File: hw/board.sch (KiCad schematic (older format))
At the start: 4 parts, among them SW1 SW_PUSH

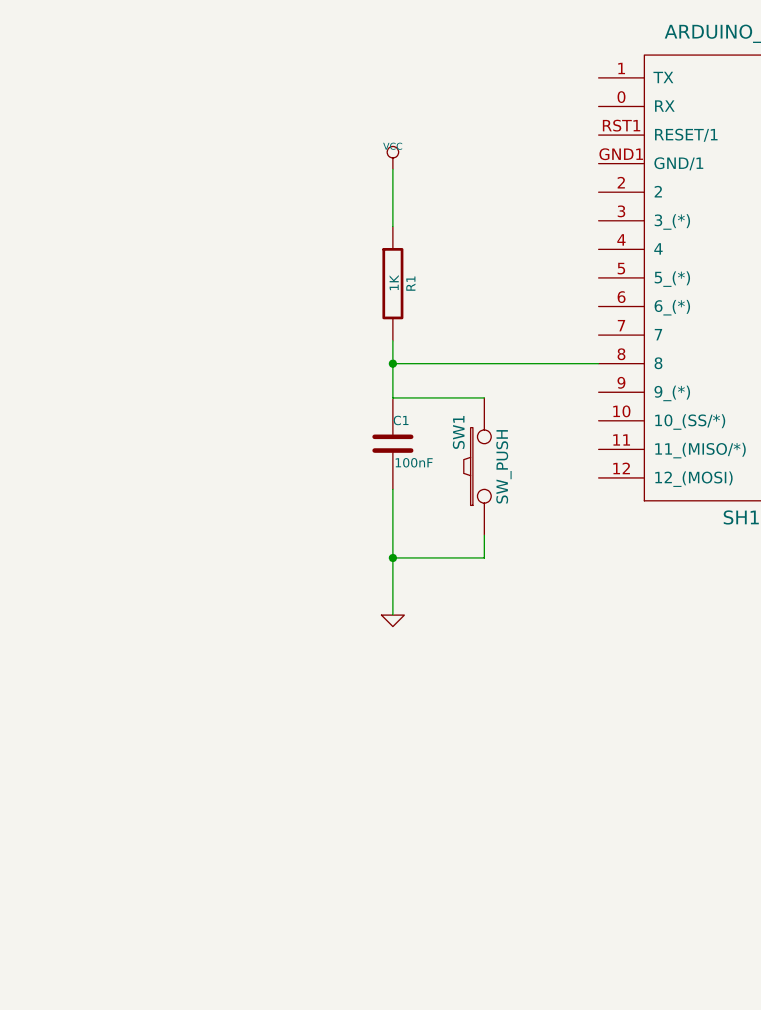
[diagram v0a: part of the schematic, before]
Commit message: Schematic update
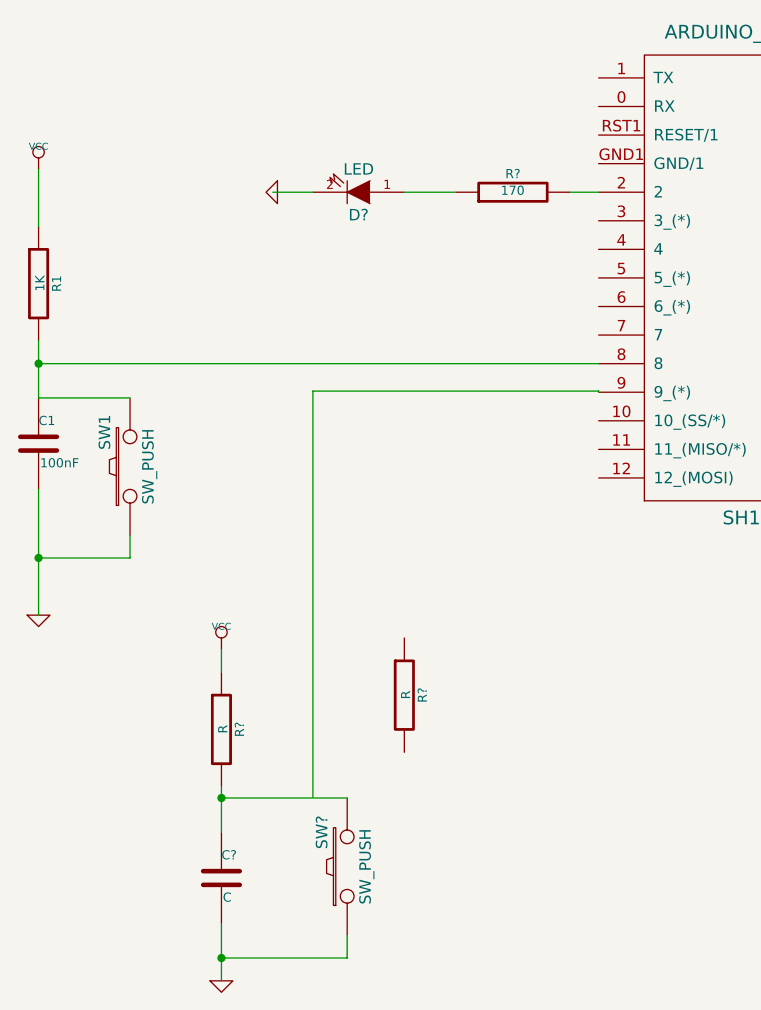
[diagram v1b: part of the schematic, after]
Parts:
- added C?: C, ~, symbol C
- added D?: LED, ~, symbol LED
- added R? (x2): R, ~, symbol R
- added R?: 170, ~, symbol R
- added SW?: SW_PUSH, ~, symbol SW_PUSH
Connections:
- wire segments 7 -> 19
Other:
- moved on the sheet: C1, R1, SW1
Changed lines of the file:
@@
 EESchema Schematic File Version 2
+LIBS:shield_arduino
 LIBS:power
 LIBS:device
@@
 LIBS:contrib
 LIBS:valves
-LIBS:shield_arduino
+LIBS:board-cache
 EELAYER 27 0
 EELAYER END
@@
 Sheet 1 1
 Title ""
-Date "19 sep 2015"
+Date "21 sep 2015"
 Rev ""
 Comp ""
@@
 L R R1
 U 1 1 55FD3C19
-P 3900 3750
-F 0 "R1" V 3980 3750 40  0000 C CNN
-F 1 "1K" V 3907 3751 40  0000 C CNN
-F 2 "~" V 3830 3750 30  0000 C CNN
-F 3 "~" H 3900 3750 30  0000 C CNN
-	1    3900 3750
+P 2350 3750
+F 0 "R1" V 2430 3750 40  0000 C CNN
+F 1 "1K" V 2357 3751 40  0000 C CNN
+F 2 "~" V 2280 3750 30  0000 C CNN
+F 3 "~" H 2350 3750 30  0000 C CNN
+	1    2350 3750
 	1    0    0    -1
 $EndComp
@@
 L C C1
 U 1 1 55FD3C28
-P 3900 4450
-F 0 "C1" H 3900 4550 40  0000 L CNN
-F 1 "100nF" H 3906 4365 40  0000 L CNN
-F 2 "~" H 3938 4300 30  0000 C CNN
-F 3 "~" H 3900 4450 60  0000 C CNN
-	1    3900 4450
+P 2350 4450
+F 0 "C1" H 2350 4550 40  0000 L CNN
+F 1 "100nF" H 2356 4365 40  0000 L CNN
+F 2 "~" H 2388 4300 30  0000 C CNN
+F 3 "~" H 2350 4450 60  0000 C CNN
+	1    2350 4450
 	1    0    0    -1
 $EndComp
@@
 L SW_PUSH SW1
 U 1 1 55FD3C5B
-P 4300 4550
-F 0 "SW1" H 4450 4660 50  0000 C CNN
-F 1 "SW_PUSH" H 4300 4470 50  0000 C CNN
-F 2 "~" H 4300 4550 60  0000 C CNN
-F 3 "~" H 4300 4550 60  0000 C CNN
-	1    4300 4550
+P 2750 4550
+F 0 "SW1" H 2900 4660 50  0000 C CNN
+F 1 "SW_PUSH" H 2750 4470 50  0000 C CNN
+F 2 "~" H 2750 4550 60  0000 C CNN
+F 3 "~" H 2750 4550 60  0000 C CNN
+	1    2750 4550
 	0    -1   -1   0
 $EndComp
@@
 L GND #PWR2
 U 1 1 55FD3C70
-P 3900 5200
-F 0 "#PWR2" H 3900 5200 30  0001 C CNN
-F 1 "GND" H 3900 5130 30  0001 C CNN
-F 2 "" H 3900 5200 60  0000 C CNN
-F 3 "" H 3900 5200 60  0000 C CNN
-	1    3900 5200
+P 2350 5200
+F 0 "#PWR2" H 2350 5200 30  0001 C CNN
+F 1 "GND" H 2350 5130 30  0001 C CNN
+F 2 "" H 2350 5200 60  0000 C CNN
+F 3 "" H 2350 5200 60  0000 C CNN
+	1    2350 5200
 	1    0    0    -1
 $EndComp
@@
 L VCC #PWR1
 U 1 1 55FD3C7F
-P 3900 3250
-F 0 "#PWR1" H 3900 3350 30  0001 C CNN
-F 1 "VCC" H 3900 3350 30  0000 C CNN
-F 2 "" H 3900 3250 60  0000 C CNN
-F 3 "" H 3900 3250 60  0000 C CNN
-	1    3900 3250
-	1    0    0    -1
-$EndComp
-Wire Wire Line
-	4300 4250 3900 4250
-Wire Wire Line
-	3900 4250 3900 4000
-Wire Wire Line
-	3900 3500 3900 3250
-Wire Wire Line
-	3900 4650 3900 5200
-Wire Wire Line
-	4300 4850 4300 4950
-Wire Wire Line
-	4300 4950 3900 4950
-Connection ~ 3900 4950
-Wire Wire Line
-	4800 4100 3900 4100
-Connection ~ 3900 4100
+P 2350 3250
+F 0 "#PWR1" H 2350 3350 30  0001 C CNN
+F 1 "VCC" H 2350 3350 30  0000 C CNN
+F 2 "" H 2350 3250 60  0000 C CNN
+F 3 "" H 2350 3250 60  0000 C CNN
+	1    2350 3250
+	1    0    0    -1
+$EndComp
+Wire Wire Line
+	2750 4250 2350 4250
+Wire Wire Line
+	2350 4250 2350 4000
+Wire Wire Line
+	2350 3500 2350 3250
+Wire Wire Line
+	2350 4650 2350 5200
+Wire Wire Line
+	2750 4850 2750 4950
+Wire Wire Line
+	2750 4950 2350 4950
+Connection ~ 2350 4950
+Connection ~ 2350 4100
+Wire Wire Line
+	2350 4100 4800 4100
+$Comp
+L R R?
+U 1 1 55FFADEF
+P 3950 5550
+F 0 "R?" V 4030 5550 40  0000 C CNN
+F 1 "R" V 3957 5551 40  0000 C CNN
+F 2 "~" V 3880 5550 30  0000 C CNN
+F 3 "~" H 3950 5550 30  0000 C CNN
+	1    3950 5550
+	1    0    0    -1
+$EndComp
+$Comp
+L R R?
+U 1 1 55FFADFE
+P 3150 5700
+F 0 "R?" V 3230 5700 40  0000 C CNN
+F 1 "R" V 3157 5701 40  0000 C CNN
+F 2 "~" V 3080 5700 30  0000 C CNN
+F 3 "~" H 3150 5700 30  0000 C CNN
+	1    3150 5700
+	1    0    0    -1
+$EndComp
+$Comp
+L C C?
+U 1 1 55FFAE0D
+P 3150 6350
+F 0 "C?" H 3150 6450 40  0000 L CNN
+F 1 "C" H 3156 6265 40  0000 L CNN
+F 2 "~" H 3188 6200 30  0000 C CNN
+F 3 "~" H 3150 6350 60  0000 C CNN
+	1    3150 6350
+	1    0    0    -1
+$EndComp
+$Comp
+L SW_PUSH SW?
+U 1 1 55FFAE33
+P 3700 6300
+F 0 "SW?" H 3850 6410 50  0000 C CNN
+F 1 "SW_PUSH" H 3700 6220 50  0000 C CNN
+F 2 "~" H 3700 6300 60  0000 C CNN
+F 3 "~" H 3700 6300 60  0000 C CNN
+	1    3700 6300
+	0    -1   -1   0
+$EndComp
+$Comp
+L VCC #PWR?
+U 1 1 55FFAE77
+P 3150 5350
+F 0 "#PWR?" H 3150 5450 30  0001 C CNN
+F 1 "VCC" H 3150 5450 30  0000 C CNN
+F 2 "" H 3150 5350 60  0000 C CNN
+F 3 "" H 3150 5350 60  0000 C CNN
+	1    3150 5350
+	1    0    0    -1
+$EndComp
+$Comp
+L GND #PWR?
+U 1 1 55FFAE8C
+P 3150 6800
+F 0 "#PWR?" H 3150 6800 30  0001 C CNN
+F 1 "GND" H 3150 6730 30  0001 C CNN
+F 2 "" H 3150 6800 60  0000 C CNN
+F 3 "" H 3150 6800 60  0000 C CNN
+	1    3150 6800
+	1    0    0    -1
+$EndComp
+Wire Wire Line
+	3150 5350 3150 5450
+Wire Wire Line
+	3150 5950 3150 6150
+Wire Wire Line
+	3150 6550 3150 6800
+Wire Wire Line
+	3700 6000 3150 6000
+Connection ~ 3150 6000
+Wire Wire Line
+	3700 6600 3700 6700
+Wire Wire Line
+	3700 6700 3150 6700
+Connection ~ 3150 6700
+Wire Wire Line
+	3550 5995 3550 4220
+Wire Wire Line
+	3550 4220 4800 4220
+Wire Wire Line
+	4800 4220 4800 4225
+$Comp
+L GND #PWR?
+U 1 1 55FFAFE2
+P 3395 3350
+F 0 "#PWR?" H 3395 3350 30  0001 C CNN
+F 1 "GND" H 3395 3280 30  0001 C CNN
+F 2 "" H 3395 3350 60  0000 C CNN
+F 3 "" H 3395 3350 60  0000 C CNN
+	1    3395 3350
+	0    1    1    0
+$EndComp
+$Comp
+L LED D?
+U 1 1 55FFB090
+P 3750 3350
+F 0 "D?" H 3750 3450 50  0000 C CNN
+F 1 "LED" H 3750 3250 50  0000 C CNN
+F 2 "~" H 3750 3350 60  0000 C CNN
+F 3 "~" H 3750 3350 60  0000 C CNN
+	1    3750 3350
+	-1   0    0    1
+$EndComp
+$Comp
+L R R?
+U 1 1 55FFB09F
+P 4425 3350
+F 0 "R?" V 4505 3350 40  0000 C CNN
+F 1 "170" V 4432 3351 40  0000 C CNN
+F 2 "~" V 4355 3350 30  0000 C CNN
+F 3 "~" H 4425 3350 30  0000 C CNN
+	1    4425 3350
+	0    -1   -1   0
+$EndComp
+Wire Wire Line
+	4800 3350 4675 3350
+Wire Wire Line
+	4175 3350 3950 3350
+Wire Wire Line
+	3375 3350 3550 3350
 $EndSCHEMATC

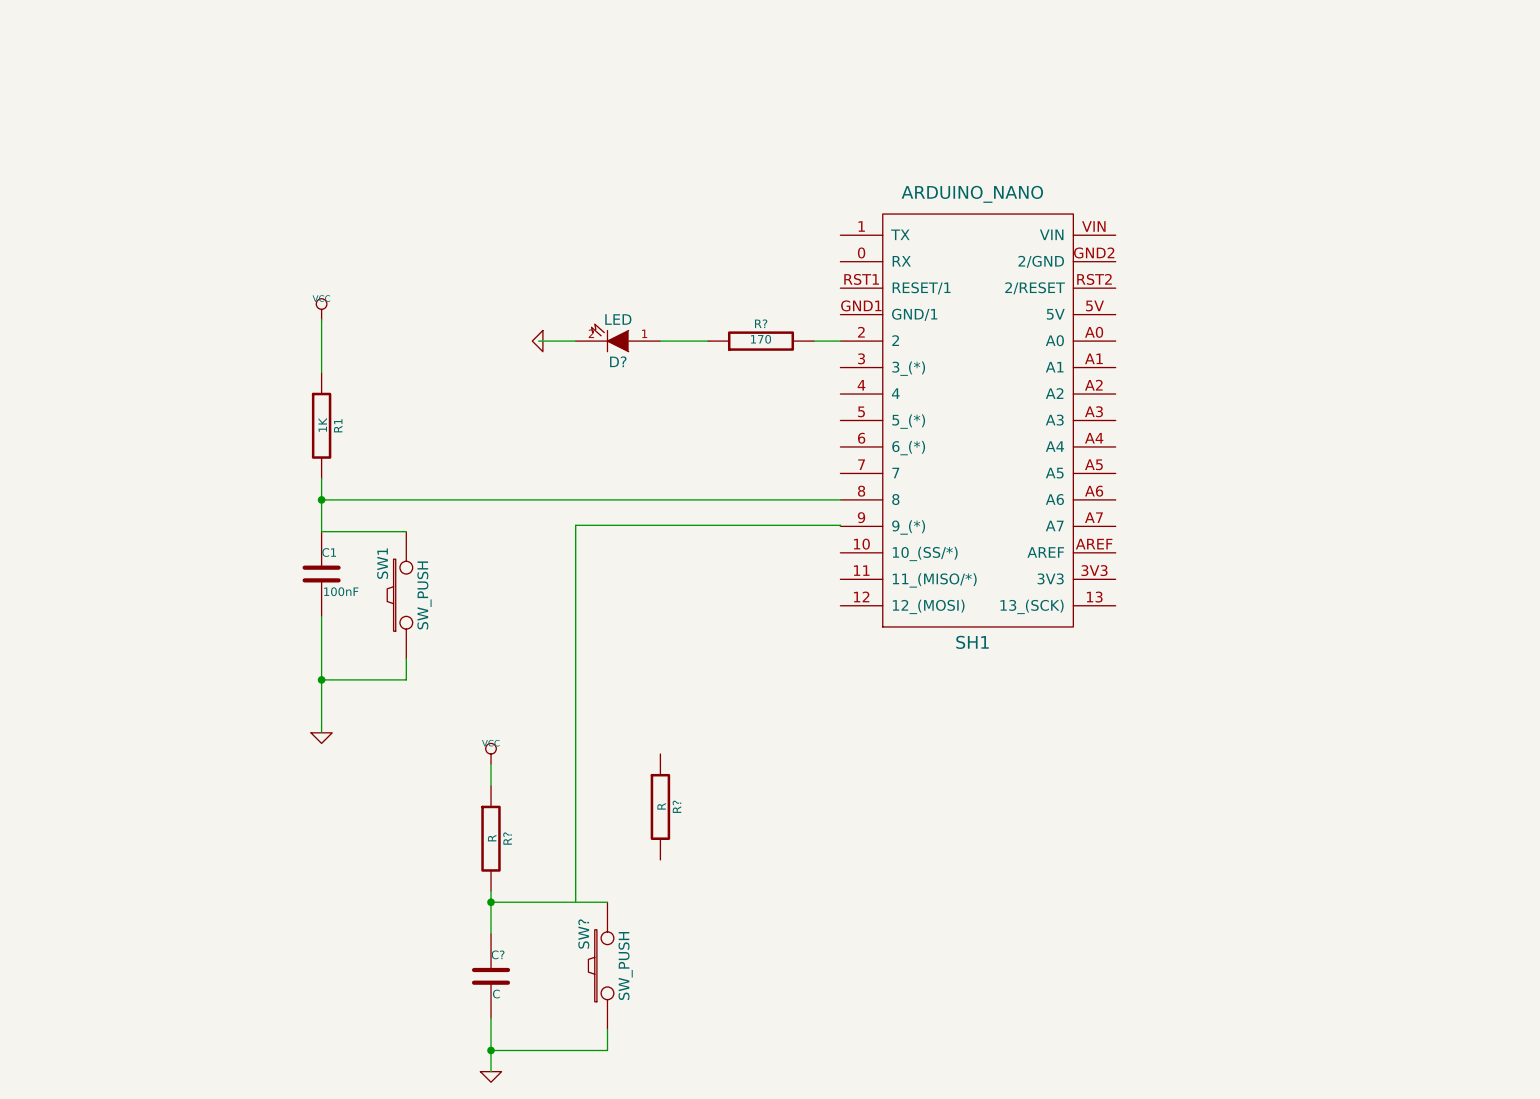
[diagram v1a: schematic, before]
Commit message: Transmitter schematic update
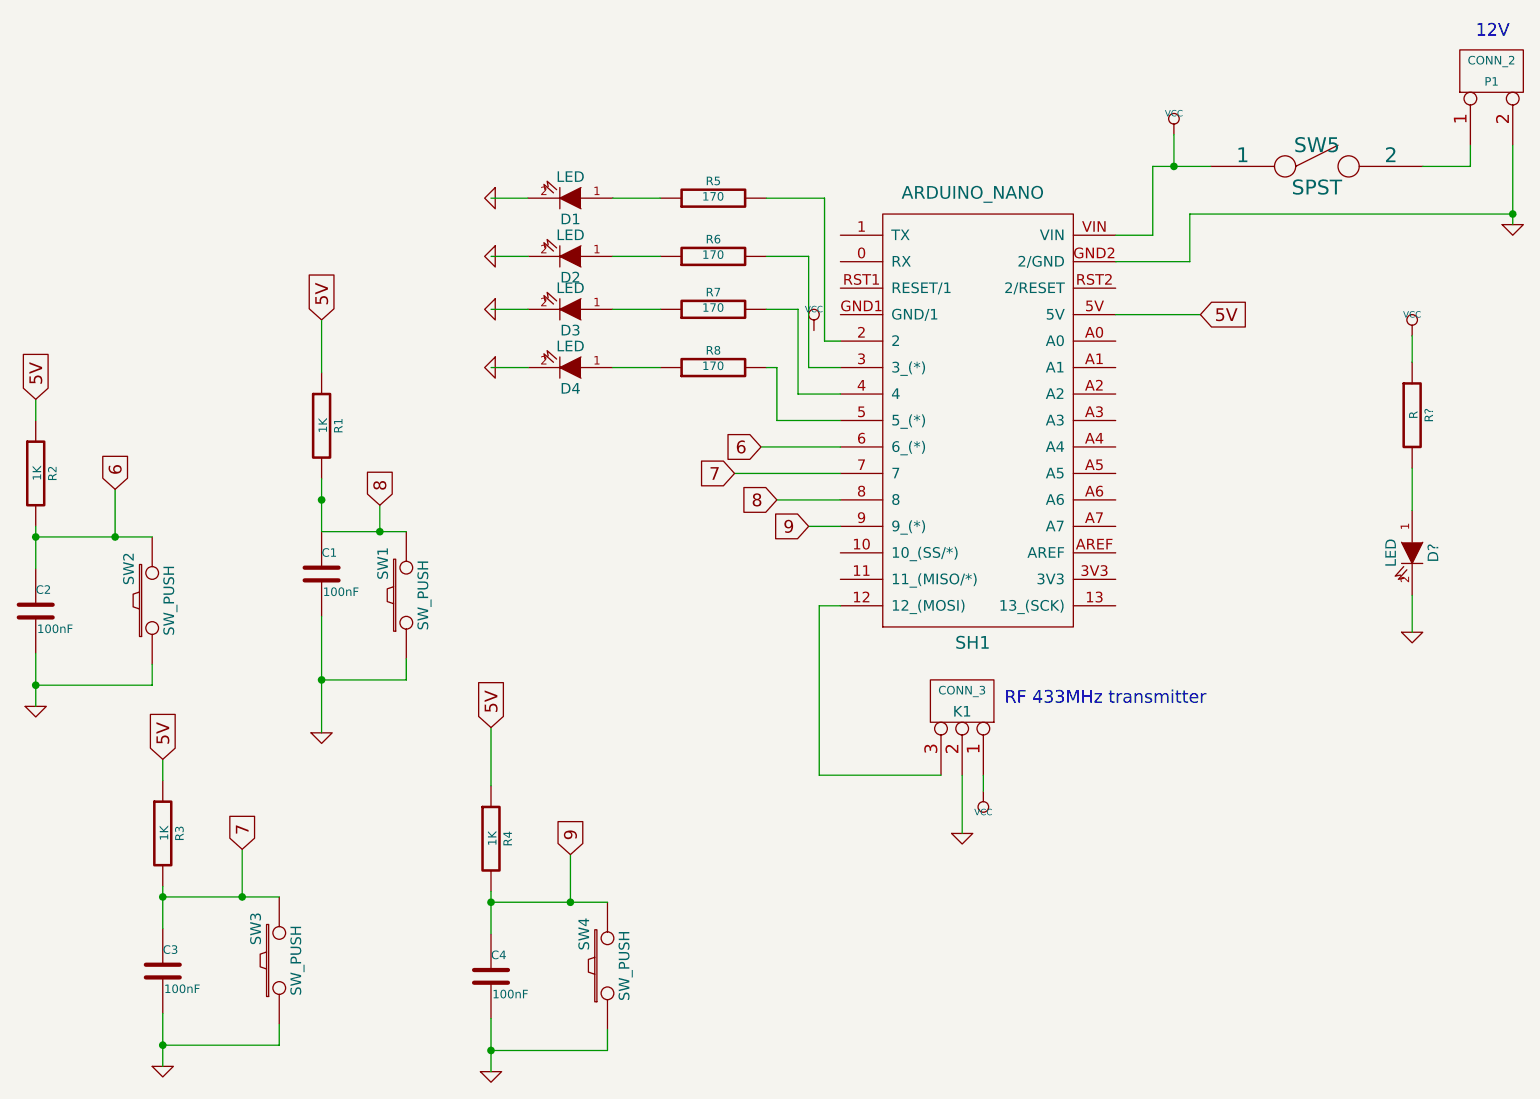
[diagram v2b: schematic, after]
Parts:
- removed R?: R, ~, symbol R
- added C2, C3: 100nF, ~, symbol C
- added D2, D3, D4, D?: LED, ~, symbol LED
- added K1: CONN_3, symbol CONN_3
- added P1: CONN_2, symbol CONN_2
- added R2, R3: 1K, ~, symbol R
- added R6, R7, R8: 170, ~, symbol R
- added R?: R, ~, symbol R
- added SW2, SW3: SW_PUSH, ~, symbol SW_PUSH
- added SW5: SPST, ~, symbol SPST
- C4: renamed from C?; value C -> 100nF
- R4: renamed from R?; value R -> 1K
- gave numbers to parts that had none: 3
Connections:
- net labels added: 5V, 6, 7, 8, 9
- wire segments 19 -> 71
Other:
- note added: "12V"
- note added: "RF 433MHz transmitter"
- moved on the sheet: D1, R5

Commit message: Adding HW schematic and correct selection of /dev/ttyUSB for arduino
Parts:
- C1, C2, C3, C4: symbol C -> C-RESCUE-board
- D1, D2, D3, D4, D?: symbol LED -> LED-RESCUE-board
- R1, R2, R3, R4, R5, R6, R7, R8, R?: symbol R -> R-RESCUE-board
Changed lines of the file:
@@
 EESchema Schematic File Version 2
-LIBS:shield_arduino
+LIBS:board-rescue
 LIBS:power
 LIBS:device
@@
 LIBS:memory
 LIBS:xilinx
-LIBS:special
 LIBS:microcontrollers
 LIBS:dsp
@@
 LIBS:contrib
 LIBS:valves
+LIBS:shield_arduino
 LIBS:board-cache
-EELAYER 27 0
+EELAYER 25 0
 EELAYER END
 $Descr A4 11693 8268
@@
 $EndComp
 $Comp
-L R R1
+L R-RESCUE-board R1
 U 1 1 55FD3C19
 P 2350 3750
@@
 $EndComp
 $Comp
-L C C1
+L C-RESCUE-board C1
 U 1 1 55FD3C28
 P 2350 4450
@@
 $EndComp
 $Comp
-L GND #PWR01
+L GND-RESCUE-board #PWR01
 U 1 1 55FD3C70
 P 2350 5200
@@
 Connection ~ 2350 4100
 $Comp
-L R R4
+L R-RESCUE-board R4
 U 1 1 55FFADFE
 P 3150 5700
@@
 $EndComp
 $Comp
-L C C4
+L C-RESCUE-board C4
 U 1 1 55FFAE0D
 P 3150 6350
@@
 $EndComp
 $Comp
-L GND #PWR02
+L GND-RESCUE-board #PWR02
 U 1 1 55FFAE8C
 P 3150 6800
@@
 Connection ~ 3150 6700
 $Comp
-L GND #PWR03
+L GND-RESCUE-board #PWR03
 U 1 1 55FFAFE2
 P 3170 2675
@@
 $EndComp
 $Comp
-L LED D1
+L LED-RESCUE-board D1
 U 1 1 55FFB090
 P 3525 2675
@@
 $EndComp
 $Comp
-L R R5
+L R-RESCUE-board R5
 U 1 1 55FFB09F
 P 4200 2675
@@
 Connection ~ 2625 4250
 $Comp
-L R R3
+L R-RESCUE-board R3
 U 1 1 56000B5A
 P 1600 5675
@@
 $EndComp
 $Comp
-L C C3
+L C-RESCUE-board C3
 U 1 1 56000B60
 P 1600 6325
@@
 $EndComp
 $Comp
-L GND #PWR04
+L GND-RESCUE-board #PWR04
 U 1 1 56000B72
 P 1600 6775
@@
 	4300 3975 4800 3975
 $Comp
-L R R2
+L R-RESCUE-board R2
 U 1 1 56000BD3
 P 1000 3975
@@
 $EndComp
 $Comp
-L C C2
+L C-RESCUE-board C2
 U 1 1 56000BD9
 P 1000 4625
@@
 $EndComp
 $Comp
-L GND #PWR05
+L GND-RESCUE-board #PWR05
 U 1 1 56000BEB
 P 1000 5075
@@
 	4425 3850 4800 3850
 $Comp
-L GND #PWR06
+L GND-RESCUE-board #PWR06
 U 1 1 56000C4A
 P 3170 2950
@@
 $EndComp
 $Comp
-L LED D2
+L LED-RESCUE-board D2
 U 1 1 56000C50
 P 3525 2950
@@
 $EndComp
 $Comp
-L R R6
+L R-RESCUE-board R6
 U 1 1 56000C56
 P 4200 2950
@@
 	3150 2950 3325 2950
 $Comp
-L GND #PWR07
+L GND-RESCUE-board #PWR07
 U 1 1 56000C5E
 P 3170 3200
@@
 $EndComp
 $Comp
-L LED D3
+L LED-RESCUE-board D3
 U 1 1 56000C64
 P 3525 3200
@@
 $EndComp
 $Comp
-L R R7
+L R-RESCUE-board R7
 U 1 1 56000C6A
 P 4200 3200
@@
 	3150 3200 3325 3200
 $Comp
-L GND #PWR08
+L GND-RESCUE-board #PWR08
 U 1 1 56000C72
 P 3170 3475
@@
 $EndComp
 $Comp
-L LED D4
+L LED-RESCUE-board D4
 U 1 1 56000C78
 P 3525 3475
@@
 $EndComp
 $Comp
-L R R8
+L R-RESCUE-board R8
 U 1 1 56000C7E
 P 4200 3475
@@
 $EndComp
 $Comp
-L GND #PWR010
+L GND-RESCUE-board #PWR010
 U 1 1 56000DD2
 P 7975 2800
@@
 	4700 5400 5275 5400
 $Comp
-L GND #PWR011
+L GND-RESCUE-board #PWR011
 U 1 1 56000FFE
 P 5375 5675
@@
 $EndComp
 $Comp
-L R R?
+L R-RESCUE-board R?
 U 1 1 56001478
 P 7500 3700
@@
 $EndComp
 $Comp
-L LED D?
+L LED-RESCUE-board D?
 U 1 1 56001487
 P 7500 4350
@@
 $EndComp
 $Comp
-L GND #PWR?
+L GND-RESCUE-board #PWR?
 U 1 1 56001496
 P 7500 4725
